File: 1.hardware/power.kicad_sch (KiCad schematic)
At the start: 0 parts

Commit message: 중간 저장
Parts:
- added J6: 12V~36V conn, symbol Connector_Generic:Conn_01x02
- added U4: LM2904AYD, PCM_Package_SO_AKL:SO-8_3.9x4.9mm_P1.27mm, symbol PCM_Amplifier_Operational_AKL:LM2904AYD
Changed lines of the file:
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@@
 	(generator "eeschema")
 	(generator_version "9.0")
-	(paper "A4")
+	(paper "C")
+	(symbol
+		(lib_id "PCM_Amplifier_Operational_AKL:LM2904AYD")
+		(at 71.12 86.36 0)
+		(unit 2)
+		(exclude_from_sim no)
+		(in_bom yes)
+		(on_board yes)
+		(dnp no)
+		(fields_autoplaced yes)
+		(property "Reference" "U4"
+			(at 72.39 76.2 0)
+			(effects
+				(font
+					(size 1.27 1.27)
+				)
+			)
+		)
+		(property "Value" "LM2904AYD"
+			(at 72.39 78.74 0)
+			(effects
+				(font
+					(size 1.27 1.27)
+				)
+			)
+		)
+		(property "Footprint" "PCM_Package_SO_AKL:SO-8_3.9x4.9mm_P1.27mm"
+			(at 71.12 86.36 0)
+			(effects
+				(font
+					(size 1.27 1.27)
+				)
+				(hide yes)
+			)
+		)
+		(property "Datasheet" "https://www.tme.eu/Document/4bbc2ee098bef99fe6a484abcdbce0a4/LM2904DT.pdf"
+			(at 71.12 86.36 0)
+			(effects
+				(font
+					(size 1.27 1.27)
+				)
+				(hide yes)
+			)
+		)
+		(property "Description" "SO-8 Dual Operational Amplifier, 2mV Offset, 30μV/°C Drift, 1.1MHz GBW, Alternate KiCAD Library"
+			(at 71.12 86.36 0)
+			(effects
+				(font
+					(size 1.27 1.27)
+				)
+				(hide yes)
+			)
+		)
+		(pin "3"
+		)
+		(pin "1"
+		)
+		(pin "2"
+		)
+		(pin "8"
+		)
+		(pin "4"
+		)
+		(pin "5"
+		)
+		(pin "7"
+		)
+		(pin "6"
+		)
+		(instances
+			(project ""
+				(path "/a25adab6-a8c3-4e0e-8ba9-baac00aaa394/fa552ebf-4859-4df7-97cc-cc5957e0d3a3"
+					(reference "U4")
+					(unit 2)
+				)
+			)
+		)
+	)
+	(symbol
+		(lib_id "Connector_Generic:Conn_01x02")
+		(at 31.75 44.45 180)
+		(unit 1)
+		(exclude_from_sim no)
+		(in_bom yes)
+		(on_board yes)
+		(dnp no)
+		(fields_autoplaced yes)
+		(property "Reference" "J6"
+			(at 31.75 35.56 0)
+			(effects
+				(font
+					(size 1.27 1.27)
+				)
+			)
+		)
+		(property "Value" "12V~36V conn"
+			(at 31.75 38.1 0)
+			(effects
+				(font
+					(size 1.27 1.27)
+				)
+			)
+		)
+		(property "Footprint" ""
+			(at 31.75 44.45 0)
+			(effects
+				(font
+					(size 1.27 1.27)
+				)
+				(hide yes)
+			)
+		)
+		(property "Datasheet" "~"
+			(at 31.75 44.45 0)
+			(effects
+				(font
+					(size 1.27 1.27)
+				)
+				(hide yes)
+			)
+		)
+		(property "Description" "Generic connector, single row, 01x02, script generated (kicad-library-utils/schlib/autogen/connector/)"
+			(at 31.75 44.45 0)
+			(effects
+				(font
+					(size 1.27 1.27)
+				)
+				(hide yes)
+			)
+		)
+		(pin "1"
+		)
+		(pin "2"
+		)
+		(instances
+			(project "bldc_motor_controller"
+				(path "/a25adab6-a8c3-4e0e-8ba9-baac00aaa394/fa552ebf-4859-4df7-97cc-cc5957e0d3a3"
+					(reference "J6")
+					(unit 1)
+				)
+			)
+		)
+	)
+	(symbol
+		(lib_id "PCM_Amplifier_Operational_AKL:LM2904AYD")
+		(at 53.34 77.47 0)
+		(unit 1)
+		(exclude_from_sim no)
+		(in_bom yes)
+		(on_board yes)
+		(dnp no)
+		(fields_autoplaced yes)
+		(property "Reference" "U4"
+			(at 66.04 71.0498 0)
+			(effects
+				(font
+					(size 1.27 1.27)
+				)
+			)
+		)
+		(property "Value" "LM2904AYD"
+			(at 66.04 73.5898 0)
+			(effects
+				(font
+					(size 1.27 1.27)
+				)
+			)
+		)
+		(property "Footprint" "PCM_Package_SO_AKL:SO-8_3.9x4.9mm_P1.27mm"
+			(at 53.34 77.47 0)
+			(effects
+				(font
+					(size 1.27 1.27)
+				)
+				(hide yes)
+			)
+		)
+		(property "Datasheet" "https://www.tme.eu/Document/4bbc2ee098bef99fe6a484abcdbce0a4/LM2904DT.pdf"
+			(at 53.34 77.47 0)
+			(effects
+				(font
+					(size 1.27 1.27)
+				)
+				(hide yes)
+			)
+		)
+		(property "Description" "SO-8 Dual Operational Amplifier, 2mV Offset, 30μV/°C Drift, 1.1MHz GBW, Alternate KiCAD Library"
+			(at 53.34 77.47 0)
+			(effects
+				(font
+					(size 1.27 1.27)
+				)
+				(hide yes)
+			)
+		)
+		(pin "3"
+		)
+		(pin "1"
+		)
+		(pin "2"
+		)
+		(pin "8"
+		)
+		(pin "4"
+		)
+		(pin "5"
+		)
+		(pin "7"
+		)
+		(pin "6"
+		)
+		(instances
+			(project ""
+				(path "/a25adab6-a8c3-4e0e-8ba9-baac00aaa394/fa552ebf-4859-4df7-97cc-cc5957e0d3a3"
+					(reference "U4")
+					(unit 1)
+				)
+			)
+		)
+	)
 )

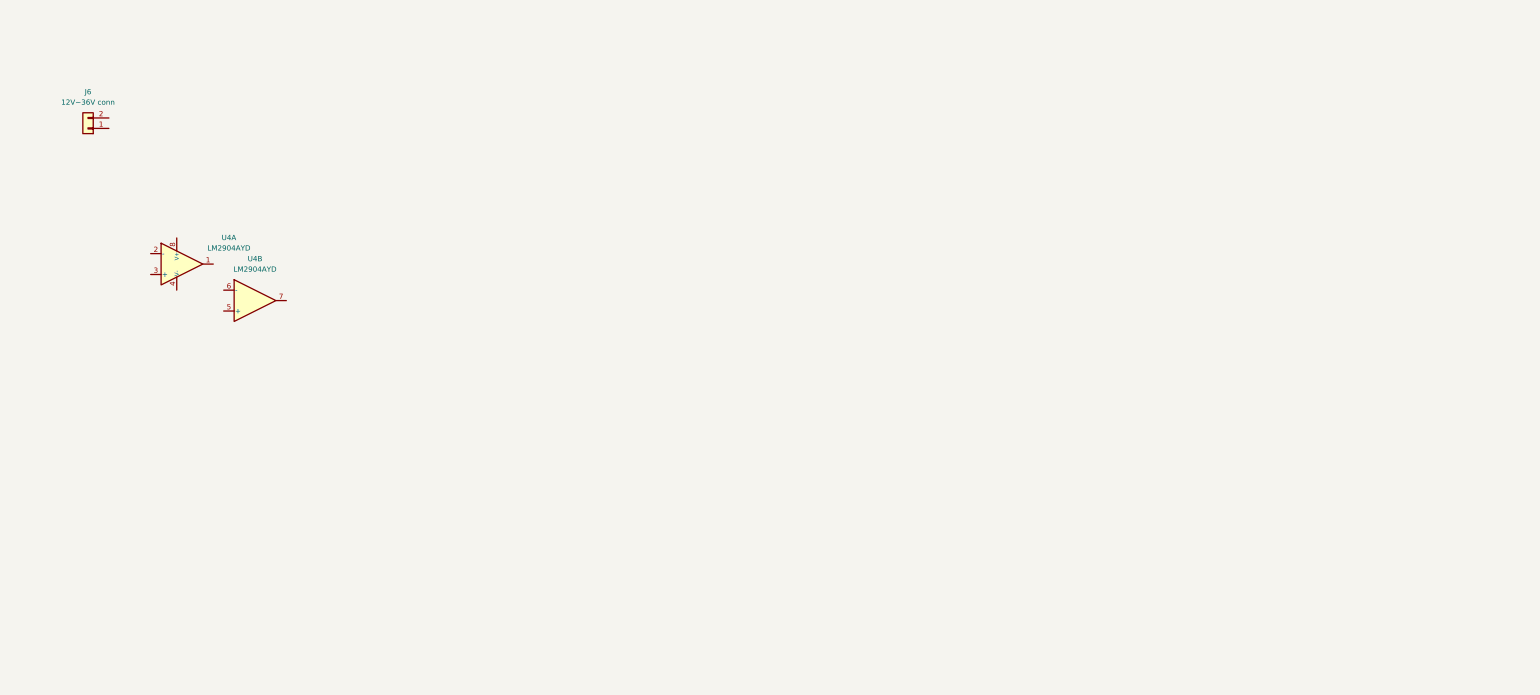
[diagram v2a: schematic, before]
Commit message: 중간저장
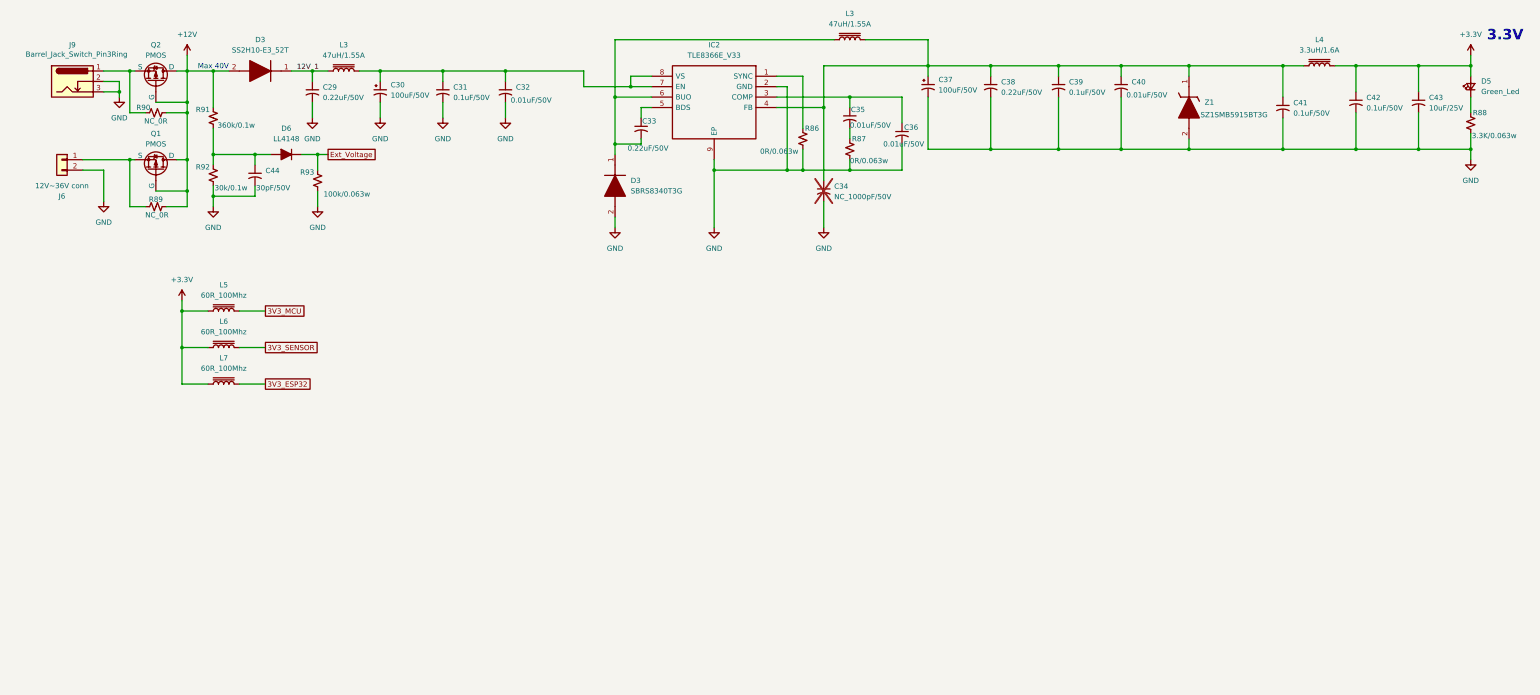
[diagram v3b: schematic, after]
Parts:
- removed U4: LM2904AYD, PCM_Package_SO_AKL:SO-8_3.9x4.9mm_P1.27mm, symbol PCM_Amplifier_Operational_AKL:LM2904AYD
- added C29, C33, C38: 0.22uF/50V, Capacitor_SMD:C_0603_1608Metric, symbol Device:C_Small_US
- added C30, C37: 100uF/50V, Capacitor_THT:CP_Radial_Tantal_D8.0mm_P5.00mm, symbol Device:C_Polarized_Small_US
- added C31, C39, C41, C42: 0.1uF/50V, Capacitor_SMD:C_0402_1005Metric, symbol Device:C_Small_US
- added C32, C35, C36, C40: 0.01uF/50V, Capacitor_SMD:C_0402_1005Metric, symbol Device:C_Small_US
- added C34: NC_1000pF/50V, Capacitor_SMD:C_0402_1005Metric, symbol Device:C_Small_US
- added C43: 10uF/25V, Capacitor_SMD:C_1206_3216Metric, symbol Device:C_Small_US
- added C44: 30pF/50V, Capacitor_SMD:C_0603_1608Metric, symbol Device:C_Small_US
- added D3: SBRS8340T3G, symbol SamacSys_Parts:SBRS8340T3G
- added D3: SS2H10-E3_52T, SamacSys_Parts:DIOM5436X244N, symbol SamacSys_Parts:SS2H10-E3_52T
- added D5: Green_Led, LED_SMD:LED_0603_1608Metric, symbol Device:LED_Small
- added D6: LL4148, PCM_Diode_SMD_AKL:D_MiniMELF, symbol PCM_Diode_AKL:LL4148
- added IC2: TLE8366E_V33, SamacSys_Parts:SOIC127P600X170-9N, symbol SamacSys_Parts:TLE8366E_V50
- added J9: Barrel_Jack_Switch_Pin3Ring, Connector_BarrelJack:BarrelJack_Wuerth_6941xx301002, symbol Connector:Barrel_Jack_Switch_Pin3Ring
- added L3 (x2): 47uH/1.55A, Inductor_SMD:L_12x12mm_H6mm, symbol Device:L_Iron
- added L4: 3.3uH/1.6A, Inductor_SMD:L_12x12mm_H6mm, symbol Device:L_Iron
- added L5, L6, L7: 60R_100Mhz, Inductor_SMD:L_0603_1608Metric, symbol Device:L_Iron
- added Q1, Q2: PMOS, symbol Simulation_SPICE:PMOS
- added R86, R87: 0R/0.063w, Resistor_SMD:R_0402_1005Metric, symbol Device:R_Small_US
- added R88: 3.3K/0.063w, Resistor_SMD:R_0402_1005Metric, symbol Device:R_Small_US
- added R89, R90: NC_0R, symbol Device:R_Small_US
- added R91: 360k/0.1w, symbol Device:R_Small_US
- added R92: 30k/0.1w, symbol Device:R_Small_US
- added R93: 100k/0.063w, symbol Device:R_Small_US
- added Z1: SZ1SMB5915BT3G, SamacSys_Parts:DIOM5436X247N, symbol SamacSys_Parts:SZ1SMB5915BT3G
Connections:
- net at J6.1 (Pin_1): now also Q1.3 (S), R89.1
- net GND: now reaches J6.2 (Pin_2)
- net GND: now also C29.2, C30.2, C31.2, C32.2, C34.2, C36.2, C37.2, C38.2, C39.2, C40.2, C41.2, C42.2, C43.2, C44.2, D3.2, IC2.2 (GND), IC2.9 (EP), J9.2, J9.3, R86.2, R87.2, R88.2, R92.1, R93.1, Z1.2
- new net: C34.1, C37.1, C38.1, C39.1, C40.1, C41.1, IC2.4 (FB), L3.2, L4.1, Z1.1
- new net: C44.1, D6.2 (A), R91.1, R92.2
- new net: C35.1, C36.1, IC2.3 (COMP)
- new net: J9.1, Q2.3 (S), R90.1
- new net: D5.1 (K), R88.1
- new net: C30.1, C31.1, C32.1, IC2.7 (EN), IC2.8 (VS), L3.2
- new net: C35.2, R87.1
- new net: C33.2, D3.1, IC2.6 (BUO), L3.1
- new net: C33.1, IC2.5 (BDS)
- new net: IC2.1 (SYNC), R86.1
- new net +12V: D3.2, Q1.1 (D), Q1.2 (G), Q2.1 (D), Q2.2 (G), R89.2, R90.2, R91.2
- new net +3.3V: C42.1, C43.1, D5.2 (A), L4.2, L5.1, L6.1, L7.1
- new net 12V_1: C29.1, D3.1, L3.1
- new net 3V3_ESP32: L7.2
- new net 3V3_MCU: L5.2
- new net 3V3_SENSOR: L6.2
- new net Ext_Voltage: D6.1 (K), R93.2
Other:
- note added: "3.3V"
- note added: "Max 40V"
- moved on the sheet: J6

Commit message: 중간 저장
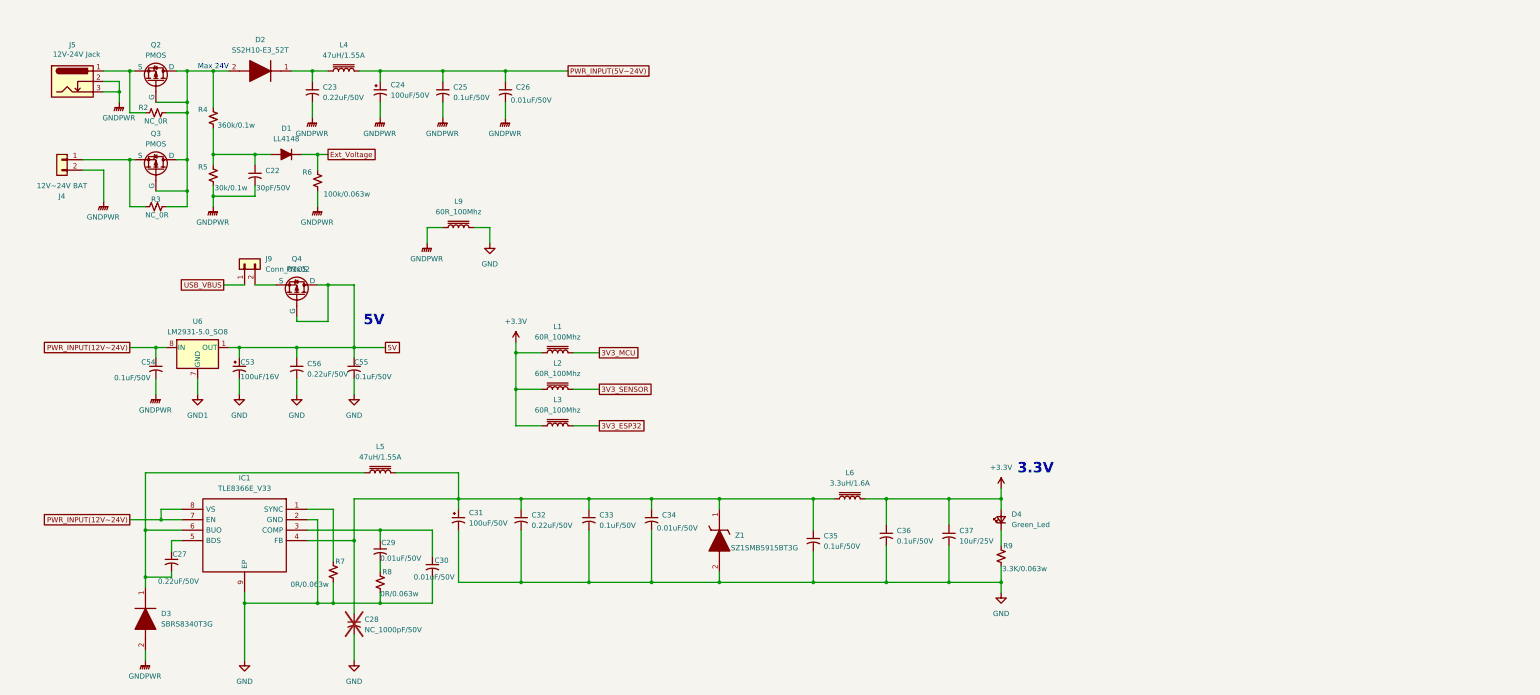
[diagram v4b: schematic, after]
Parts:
- added C53: 100uF/16V, Capacitor_THT:CP_Radial_Tantal_D8.0mm_P5.00mm, symbol Device:C_Polarized_Small_US
- added C54, C55: 0.1uF/50V, Capacitor_SMD:C_0402_1005Metric, symbol Device:C_Small_US
- added C56: 0.22uF/50V, Capacitor_SMD:C_0603_1608Metric, symbol Device:C_Small_US
- added J9: Conn_01x02, symbol Connector_Generic:Conn_01x02
- added L9: 60R_100Mhz, Inductor_SMD:L_0603_1608Metric, symbol Device:L_Iron
- added Q4: PMOS, symbol Simulation_SPICE:PMOS
- added U6: LM2931-5.0_SO8, Package_SO:SOIC-8_3.9x4.9mm_P1.27mm, symbol Regulator_Linear:LM2931-5.0_SO8
- J4: renamed from J6; value 12V~36V conn -> 12V~24V BAT
- J5: renamed from J9; value Barrel_Jack_Switch_Pin3Ring -> 12V-24V Jack
- renumbered C44 to C22, C29 to C23, C30 to C24, C31 to C25, C32 to C26, C33 to C27, C34 to C28, C35 to C29, C36 to C30, C37 to C31, C38 to C32, C39 to C33, C40 to C34, C41 to C35, C42 to C36, C43 to C37, D6 to D1, D3 to D2, D5 to D4, IC2 to IC1, L5 to L1, L6 to L2, L7 to L3, L3 to L4, L3 to L5, L4 to L6, Q1 to Q3, R90 to R2, R89 to R3, R91 to R4, R92 to R5, R93 to R6, R86 to R7, R87 to R8, R88 to R9
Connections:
- net GND: now also C53.2, C55.2, C56.2, L9.2; no longer C22.2, C23.2, C24.2, C25.2, C26.2, D3.2, J4.2 (Pin_2), J5.2, J5.3, R5.1, R6.1
- net PWR_INPUT(5V~24V): now reaches C24.1, C25.1, C26.1, L4.2
- net PWR_INPUT(5V~24V): no longer IC1.7 (EN), IC1.8 (VS)
- net +12V: no longer names the net of D2.2, Q2.1 (D), Q2.2 (G), Q3.1 (D), Q3.2 (G), R2.2, R3.2, R4.2
- net 12V_1: no longer names the net of C23.1, D2.1, L4.1
- new net: J9.2 (Pin_2), Q4.3 (S)
- new net 5V: C53.1, C55.1, C56.1, Q4.1 (D), Q4.2 (G), U6.1 (OUT)
- new net GND1: U6.2 (GND), U6.3 (GND), U6.6 (GND), U6.7 (GND)
- new net GNDPWR: C22.2, C23.2, C24.2, C25.2, C26.2, C54.2, D3.2, J4.2 (Pin_2), J5.2, J5.3, L9.1, R5.1, R6.1
- new net PWR_INPUT(12V~24V): C54.1, IC1.7 (EN), IC1.8 (VS), U6.8 (IN)
- new net USB_VBUS: J9.1 (Pin_1)
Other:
- note added: "5V"
- note added: "Max 24V"
- note removed: "Max 40V"
- moved on the sheet: C27, C28, C29, C30, C31, C32, C33, C34, C35, C36, C37, D3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

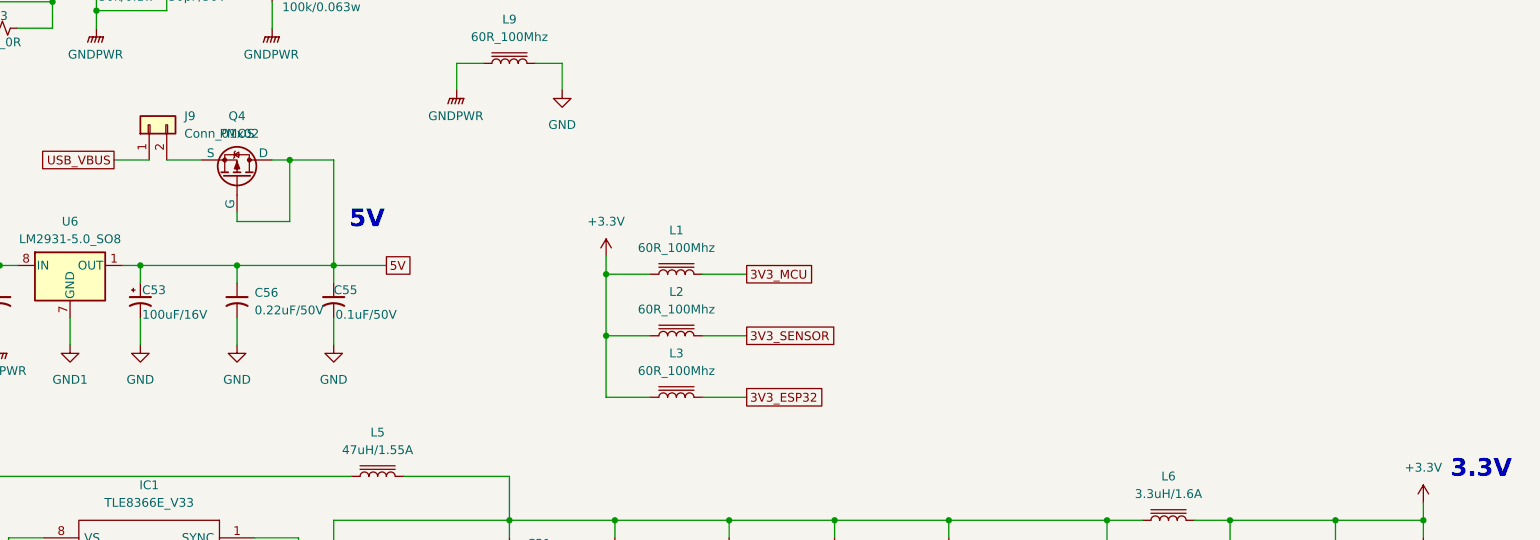
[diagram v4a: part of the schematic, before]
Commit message: 중간 저장
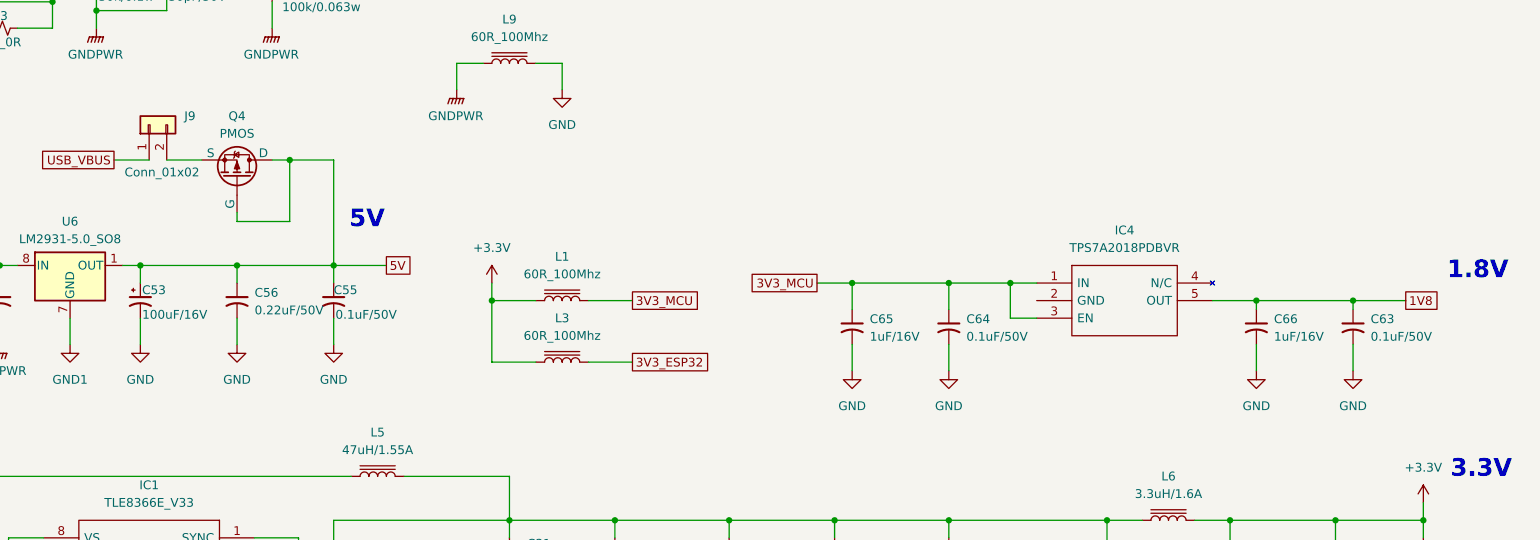
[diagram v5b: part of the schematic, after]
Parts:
- removed L2: 60R_100Mhz, Inductor_SMD:L_0603_1608Metric, symbol Device:L_Iron
- added C63, C64: 0.1uF/50V, Capacitor_SMD:C_0402_1005Metric, symbol Device:C_Small_US
- added C65, C66: 1uF/16V, Capacitor_SMD:C_0402_1005Metric, symbol Device:C_Small_US
- added IC4: TPS7A2018PDBVR, SOT95P280X145-5N, symbol SamacSys_Parts:TPS7A20185PDBVR
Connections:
- net 3V3_MCU: now also C64.1, C65.1, IC4.1 (IN), IC4.3 (EN)
- net GND: now also C63.2, C64.2, C65.2, C66.2
- new net 1V8: C63.1, C66.1, IC4.5 (OUT)
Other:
- note added: "1.8V"
- moved on the sheet: L1, L3
